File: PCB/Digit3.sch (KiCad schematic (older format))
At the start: 1 part

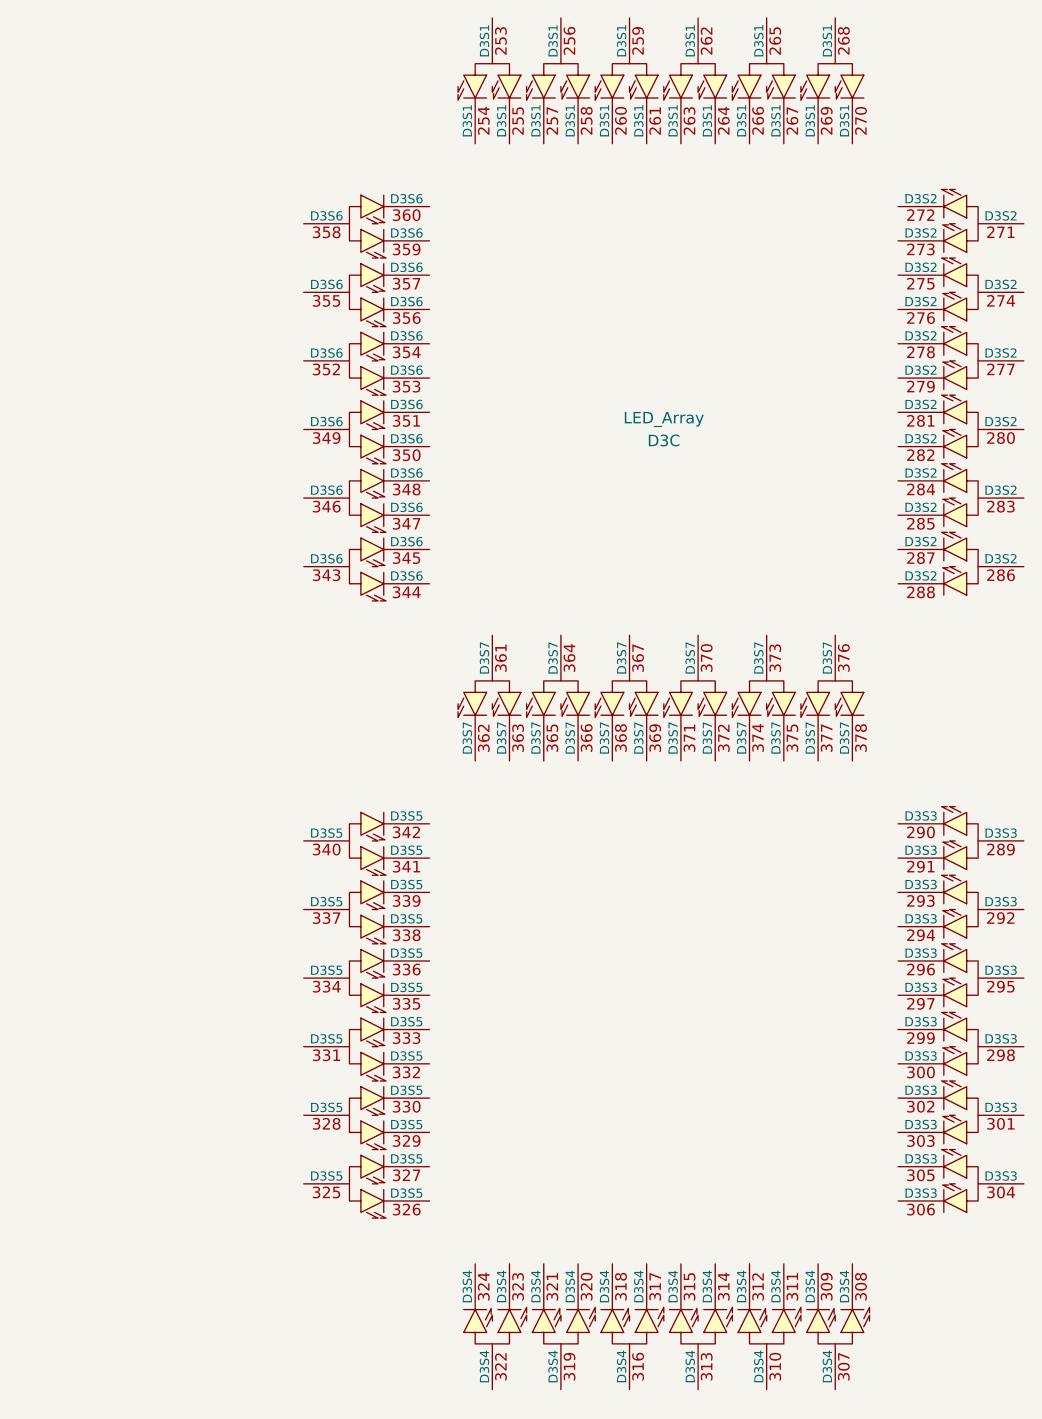
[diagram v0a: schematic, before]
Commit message: Worked on PCB.
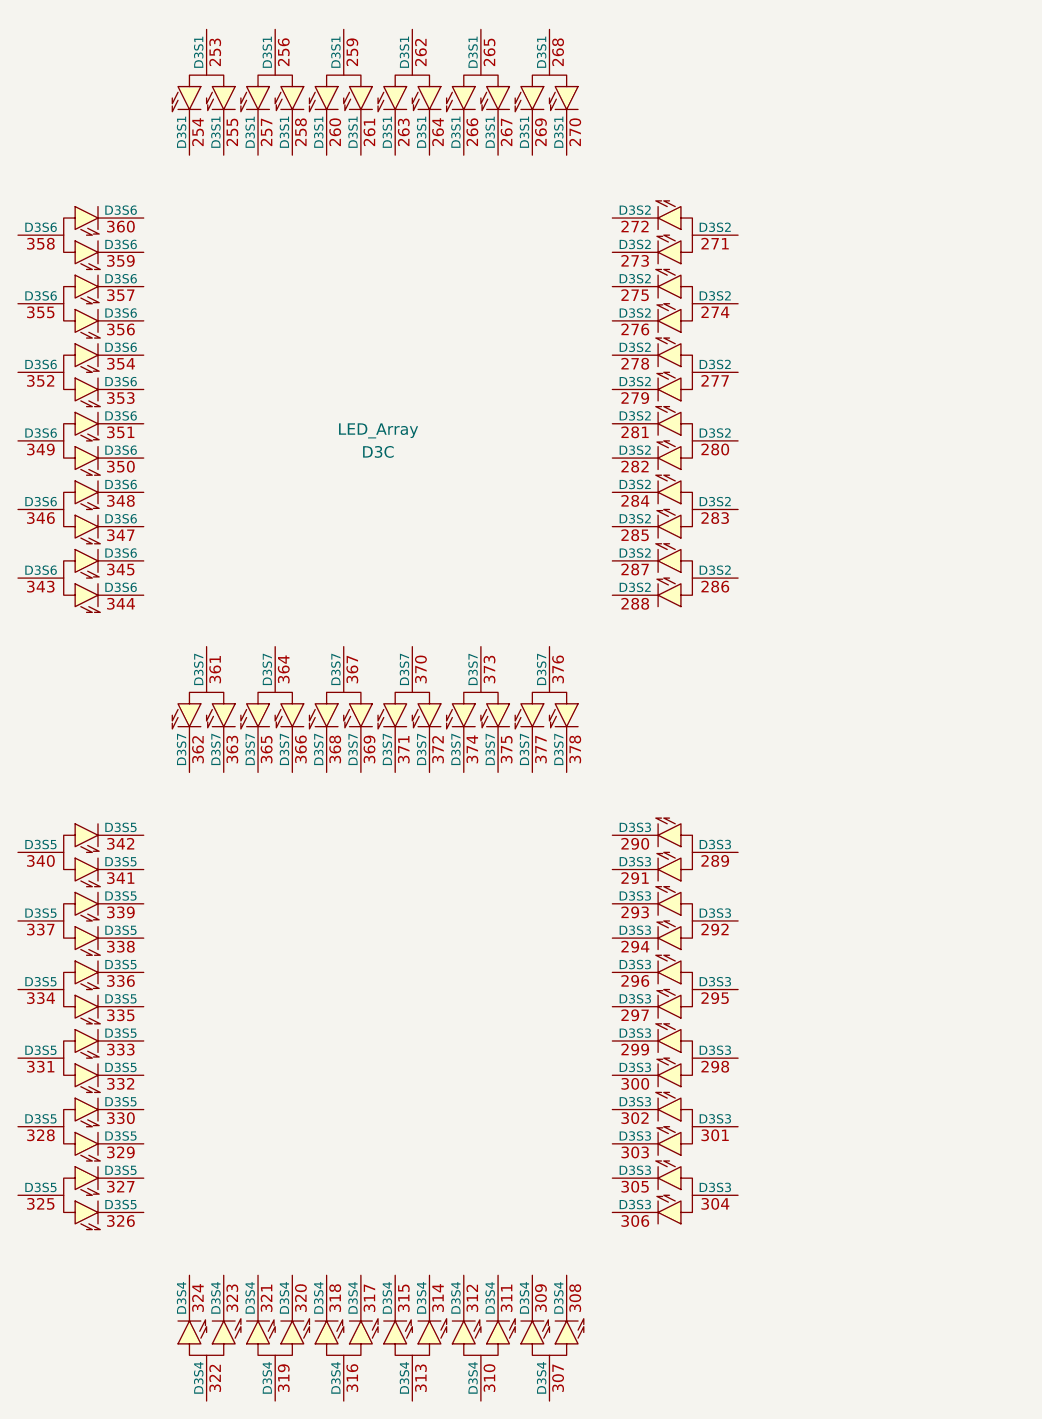
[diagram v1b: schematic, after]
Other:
- moved on the sheet: D3C
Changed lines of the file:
@@
 L LED_Array D3
 U 3 1 54BC7666
-P 5000 4100
-F 0 "D3" H 5000 5250 50  0000 C CNN
-F 1 "LED_Array" H 5000 5350 50  0000 C CNN
-F 2 "Custom:LED-ARRAY" H 5000 5025 50  0001 C CNN
-F 3 "" H 5000 5025 50  0000 C CNN
-	3    5000 4100
+P 3750 4150
+F 0 "D3" H 3750 5300 50  0000 C CNN
+F 1 "LED_Array" H 3750 5400 50  0000 C CNN
+F 2 "Custom:LED-ARRAY" H 3750 5075 50  0001 C CNN
+F 3 "" H 3750 5075 50  0000 C CNN
+	3    3750 4150
 	1    0    0    -1
 $EndComp

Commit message: Updated schematic.
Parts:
- added Q? (x14): FDG1024NZ, SC70-6, symbol FDG1024NZ
- added R? (x14): 10K, symbol R
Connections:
- net labels added: D2A1, D2A2, D2A3, D2A4, D2A5, D2A6, D2S1G, D2S1R, D2S2G, D2S2R, D2S3G, D2S3R, D2S4G, D2S4R, D2S5G, D2S5R, D2S6G, D2S6R, D2S7G, D2S7R, GND
- wire segments 0 -> 257
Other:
- moved on the sheet: D3C
